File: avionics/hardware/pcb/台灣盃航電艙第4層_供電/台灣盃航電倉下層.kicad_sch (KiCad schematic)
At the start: 42 parts, among them J1 XT60, J2 XT60, J3 Conn_01x06_Pin, J4 Pyro1, J5 Pyro2, Q1 NMOS, Q2 NMOS, Q3 NMOS, Q4 NMOS, U11 Connector, U3 LM2596S-5, U4 LM2596S-5, U5 AMS1117-3.3, U6 AMS1117-3.3

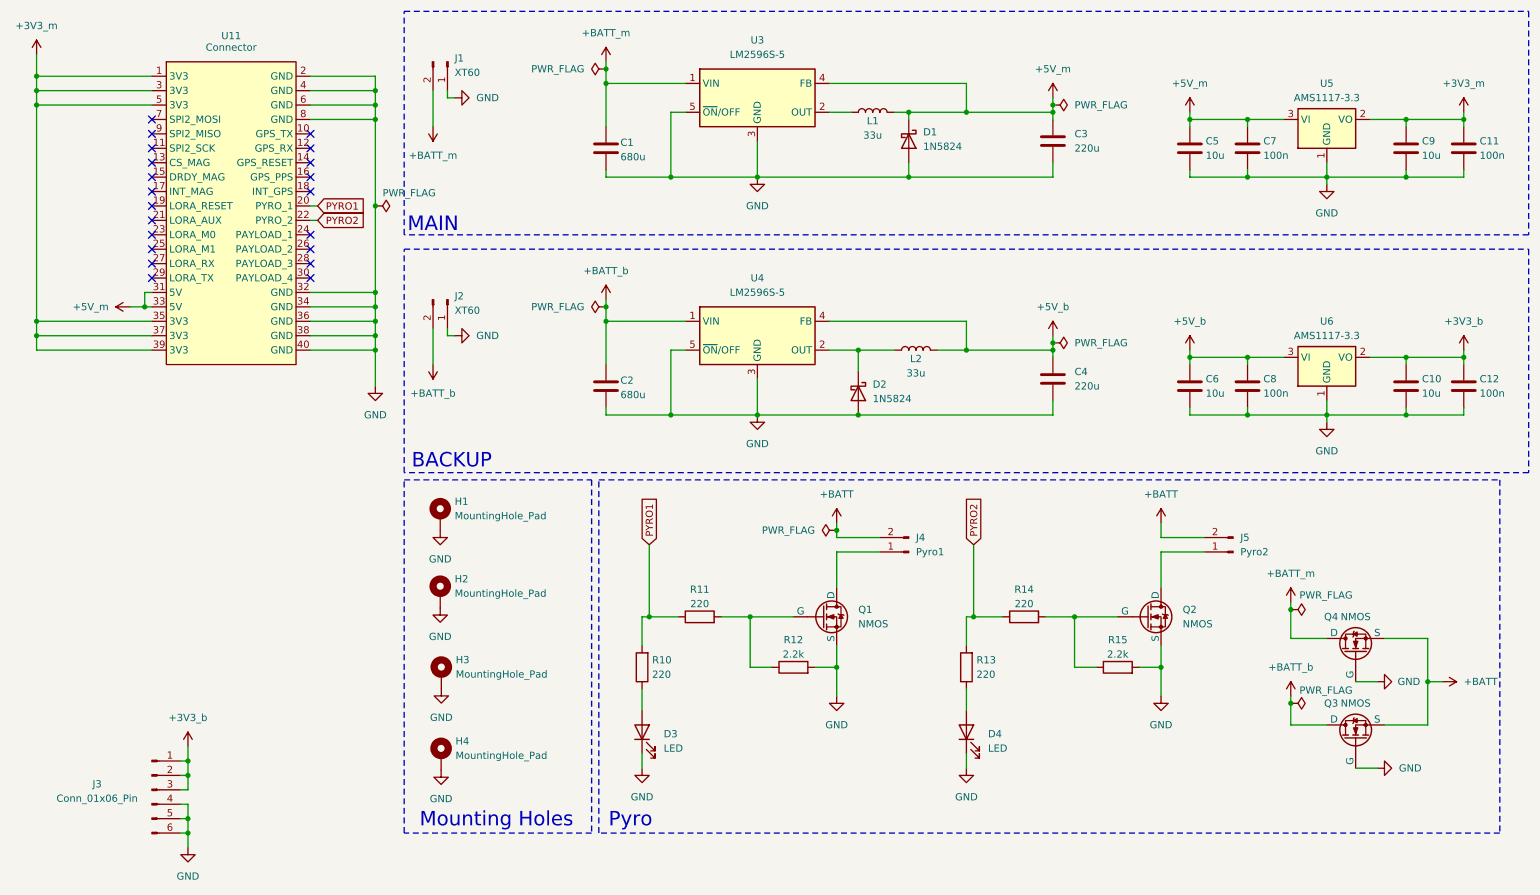
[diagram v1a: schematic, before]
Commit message: 完成PCB最終設計
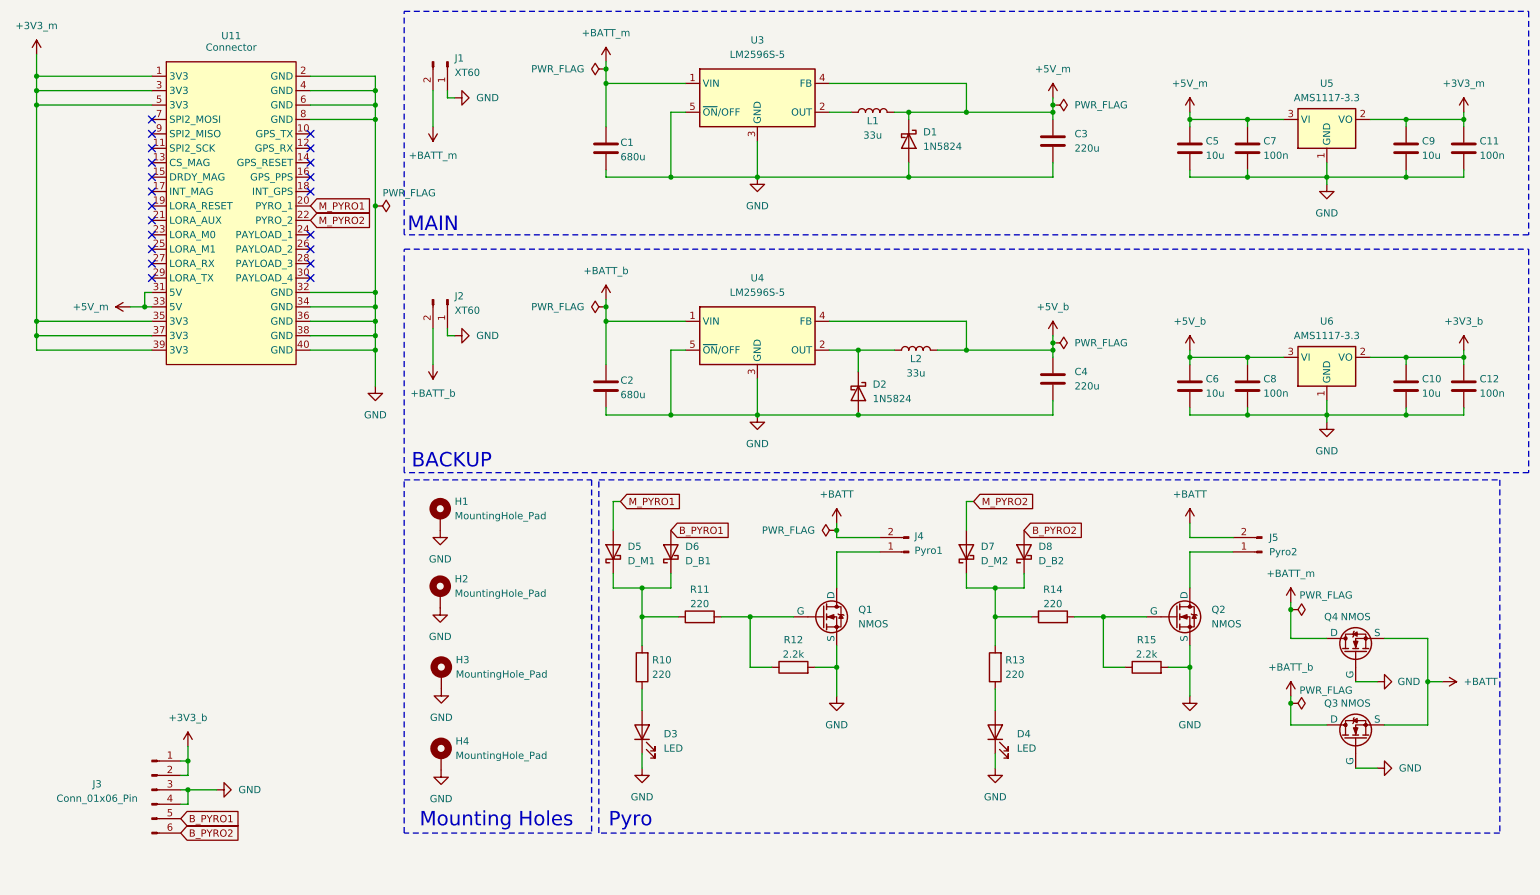
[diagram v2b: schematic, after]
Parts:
- added D5: D_M1, Diode_SMD:D_SOD-123, symbol Device:D_Schottky
- added D6: D_B1, Diode_SMD:D_SOD-123, symbol Device:D_Schottky
- added D7: D_M2, Diode_SMD:D_SOD-123, symbol Device:D_Schottky
- added D8: D_B2, Diode_SMD:D_SOD-123, symbol Device:D_Schottky
- J4, J5: footprint Connector_JST:JST_XH_B2B-XH-A_1x02_P2.50mm_Vertical -> Connector_JST:JST_XH_S2B-XH-A_1x02_P2.50mm_Horizontal
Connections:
- net +3V3_b: no longer J3.3 (Pin_3)
- net GND: now also J3.3 (Pin_3); no longer J3.5 (Pin_5), J3.6 (Pin_6)
- net PYRO1: no longer names the net of R10.2, R11.1
- net PYRO1: now also D5.1 (K), D6.1 (K); no longer U11.20 (PYRO_1)
- net PYRO2: no longer names the net of R13.2, R14.1
- net PYRO2: now also D7.1 (K), D8.1 (K); no longer U11.22 (PYRO_2)
- new net B_PYRO1: D6.2 (A), J3.5 (Pin_5)
- new net B_PYRO2: D8.2 (A), J3.6 (Pin_6)
- new net M_PYRO1: D5.2 (A), U11.20 (PYRO_1)
- new net M_PYRO2: D7.2 (A), U11.22 (PYRO_2)
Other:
- moved on the sheet: D4, J5, Q2, R13, R14, R15
